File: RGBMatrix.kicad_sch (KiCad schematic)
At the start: 208 parts

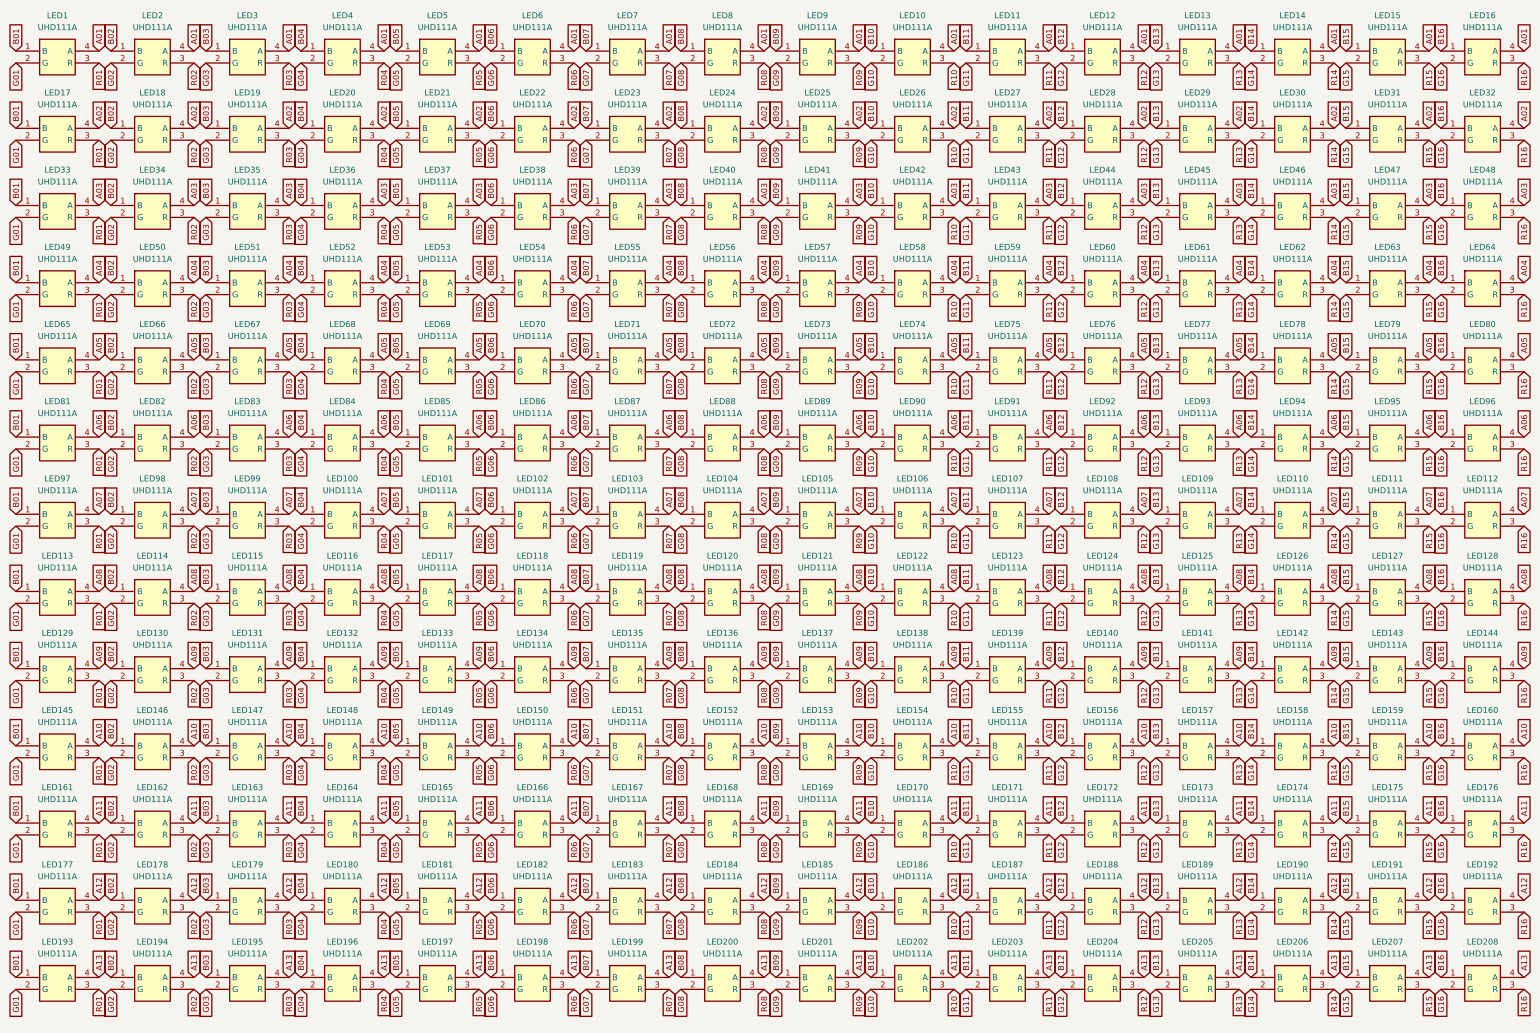
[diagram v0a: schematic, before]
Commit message: anodColumn, colorRow
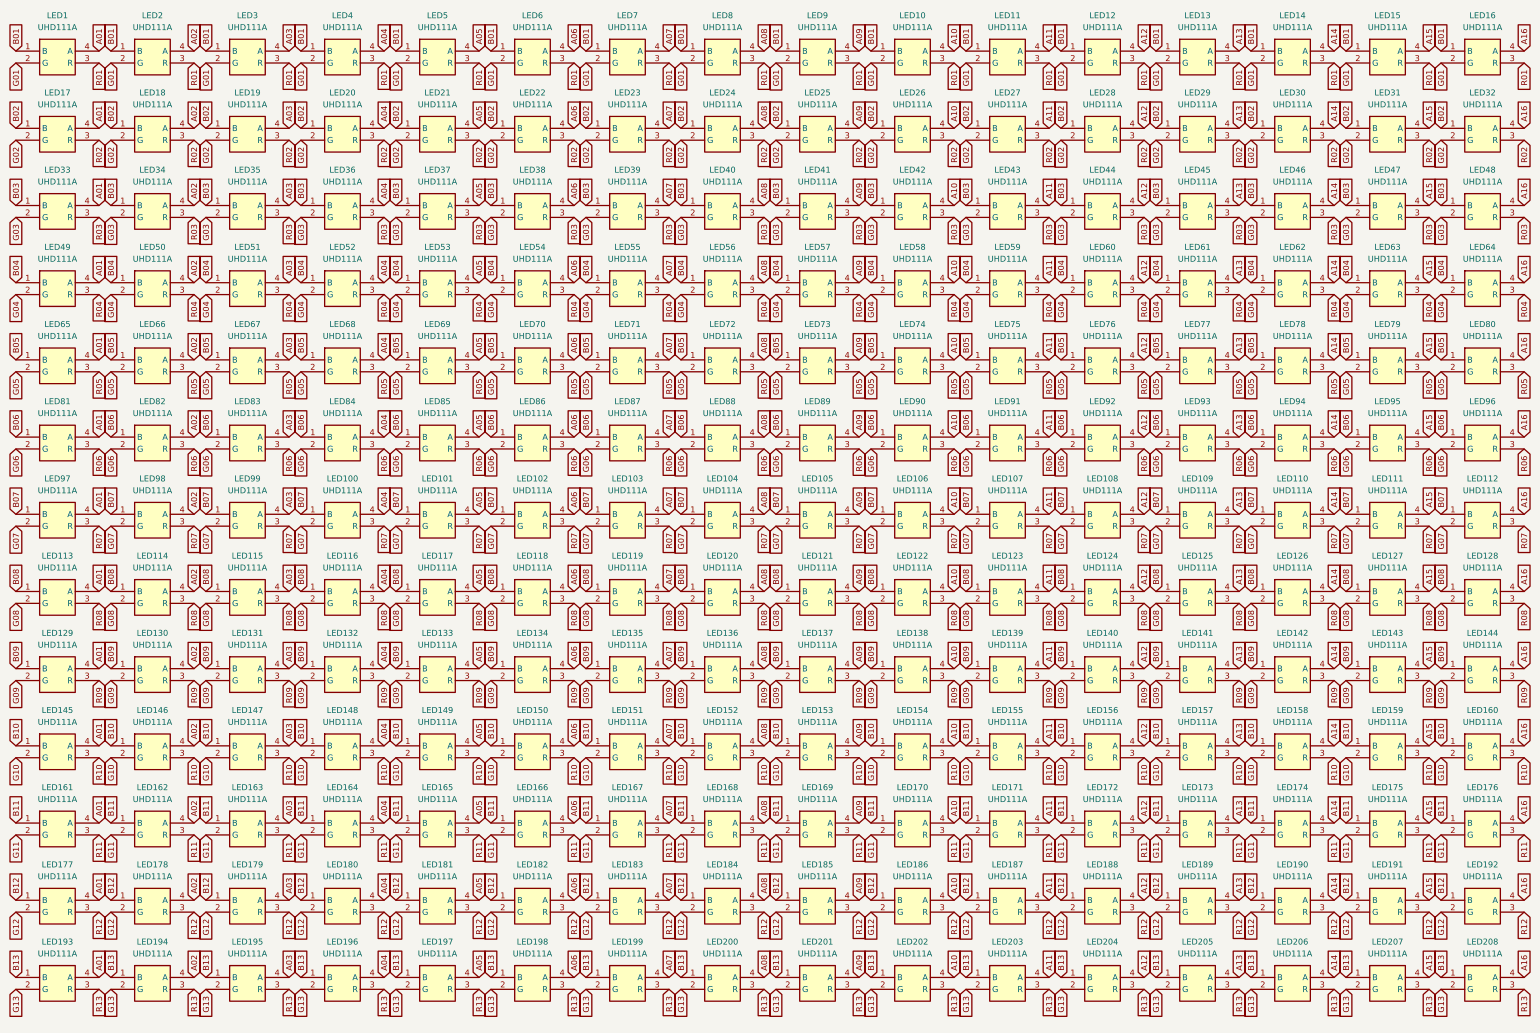
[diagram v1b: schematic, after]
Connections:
- net A01: now also LED113.4 (A), LED129.4 (A), LED145.4 (A), LED161.4 (A), LED17.4 (A), LED177.4 (A), LED193.4 (A), LED33.4 (A), LED49.4 (A), LED65.4 (A), LED81.4 (A), LED97.4 (A); no longer LED10.4 (A), LED11.4 (A), LED12.4 (A), LED13.4 (A), LED14.4 (A), LED15.4 (A), LED16.4 (A), LED2.4 (A), LED3.4 (A), LED4.4 (A), LED5.4 (A), LED6.4 (A), LED7.4 (A), LED8.4 (A), LED9.4 (A)
- net A02: now also LED114.4 (A), LED130.4 (A), LED146.4 (A), LED162.4 (A), LED178.4 (A), LED194.4 (A), LED2.4 (A), LED34.4 (A), LED50.4 (A), LED66.4 (A), LED82.4 (A), LED98.4 (A); no longer LED17.4 (A), LED19.4 (A), LED20.4 (A), LED21.4 (A), LED22.4 (A), LED23.4 (A), LED24.4 (A), LED25.4 (A), LED26.4 (A), LED27.4 (A), LED28.4 (A), LED29.4 (A), LED30.4 (A), LED31.4 (A), LED32.4 (A)
- net A03: now also LED115.4 (A), LED131.4 (A), LED147.4 (A), LED163.4 (A), LED179.4 (A), LED19.4 (A), LED195.4 (A), LED3.4 (A), LED51.4 (A), LED67.4 (A), LED83.4 (A), LED99.4 (A); no longer LED33.4 (A), LED34.4 (A), LED36.4 (A), LED37.4 (A), LED38.4 (A), LED39.4 (A), LED40.4 (A), LED41.4 (A), LED42.4 (A), LED43.4 (A), LED44.4 (A), LED45.4 (A), LED46.4 (A), LED47.4 (A), LED48.4 (A)
- net A04: now also LED100.4 (A), LED116.4 (A), LED132.4 (A), LED148.4 (A), LED164.4 (A), LED180.4 (A), LED196.4 (A), LED20.4 (A), LED36.4 (A), LED4.4 (A), LED68.4 (A), LED84.4 (A); no longer LED49.4 (A), LED50.4 (A), LED51.4 (A), LED53.4 (A), LED54.4 (A), LED55.4 (A), LED56.4 (A), LED57.4 (A), LED58.4 (A), LED59.4 (A), LED60.4 (A), LED61.4 (A), LED62.4 (A), LED63.4 (A), LED64.4 (A)
- net A05: now also LED101.4 (A), LED117.4 (A), LED133.4 (A), LED149.4 (A), LED165.4 (A), LED181.4 (A), LED197.4 (A), LED21.4 (A), LED37.4 (A), LED5.4 (A), LED53.4 (A), LED85.4 (A); no longer LED65.4 (A), LED66.4 (A), LED67.4 (A), LED68.4 (A), LED70.4 (A), LED71.4 (A), LED72.4 (A), LED73.4 (A), LED74.4 (A), LED75.4 (A), LED76.4 (A), LED77.4 (A), LED78.4 (A), LED79.4 (A), LED80.4 (A)
- net A06: now also LED102.4 (A), LED118.4 (A), LED134.4 (A), LED150.4 (A), LED166.4 (A), LED182.4 (A), LED198.4 (A), LED22.4 (A), LED38.4 (A), LED54.4 (A), LED6.4 (A), LED70.4 (A); no longer LED81.4 (A), LED82.4 (A), LED83.4 (A), LED84.4 (A), LED85.4 (A), LED87.4 (A), LED88.4 (A), LED89.4 (A), LED90.4 (A), LED91.4 (A), LED92.4 (A), LED93.4 (A), LED94.4 (A), LED95.4 (A), LED96.4 (A)
- net A07: now also LED119.4 (A), LED135.4 (A), LED151.4 (A), LED167.4 (A), LED183.4 (A), LED199.4 (A), LED23.4 (A), LED39.4 (A), LED55.4 (A), LED7.4 (A), LED71.4 (A), LED87.4 (A); no longer LED100.4 (A), LED101.4 (A), LED102.4 (A), LED104.4 (A), LED105.4 (A), LED106.4 (A), LED107.4 (A), LED108.4 (A), LED109.4 (A), LED110.4 (A), LED111.4 (A), LED112.4 (A), LED97.4 (A), LED98.4 (A), LED99.4 (A)
- net A08: now also LED104.4 (A), LED136.4 (A), LED152.4 (A), LED168.4 (A), LED184.4 (A), LED200.4 (A), LED24.4 (A), LED40.4 (A), LED56.4 (A), LED72.4 (A), LED8.4 (A), LED88.4 (A); no longer LED113.4 (A), LED114.4 (A), LED115.4 (A), LED116.4 (A), LED117.4 (A), LED118.4 (A), LED119.4 (A), LED121.4 (A), LED122.4 (A), LED123.4 (A), LED124.4 (A), LED125.4 (A), LED126.4 (A), LED127.4 (A), LED128.4 (A)
- net A09: now also LED105.4 (A), LED121.4 (A), LED153.4 (A), LED169.4 (A), LED185.4 (A), LED201.4 (A), LED25.4 (A), LED41.4 (A), LED57.4 (A), LED73.4 (A), LED89.4 (A), LED9.4 (A); no longer LED129.4 (A), LED130.4 (A), LED131.4 (A), LED132.4 (A), LED133.4 (A), LED134.4 (A), LED135.4 (A), LED136.4 (A), LED138.4 (A), LED139.4 (A), LED140.4 (A), LED141.4 (A), LED142.4 (A), LED143.4 (A), LED144.4 (A)
- net A10: now also LED10.4 (A), LED106.4 (A), LED122.4 (A), LED138.4 (A), LED170.4 (A), LED186.4 (A), LED202.4 (A), LED26.4 (A), LED42.4 (A), LED58.4 (A), LED74.4 (A), LED90.4 (A); no longer LED145.4 (A), LED146.4 (A), LED147.4 (A), LED148.4 (A), LED149.4 (A), LED150.4 (A), LED151.4 (A), LED152.4 (A), LED153.4 (A), LED155.4 (A), LED156.4 (A), LED157.4 (A), LED158.4 (A), LED159.4 (A), LED160.4 (A)
- net A11: now also LED107.4 (A), LED11.4 (A), LED123.4 (A), LED139.4 (A), LED155.4 (A), LED187.4 (A), LED203.4 (A), LED27.4 (A), LED43.4 (A), LED59.4 (A), LED75.4 (A), LED91.4 (A); no longer LED161.4 (A), LED162.4 (A), LED163.4 (A), LED164.4 (A), LED165.4 (A), LED166.4 (A), LED167.4 (A), LED168.4 (A), LED169.4 (A), LED170.4 (A), LED172.4 (A), LED173.4 (A), LED174.4 (A), LED175.4 (A), LED176.4 (A)
- net A12: now also LED108.4 (A), LED12.4 (A), LED124.4 (A), LED140.4 (A), LED156.4 (A), LED172.4 (A), LED204.4 (A), LED28.4 (A), LED44.4 (A), LED60.4 (A), LED76.4 (A), LED92.4 (A); no longer LED177.4 (A), LED178.4 (A), LED179.4 (A), LED180.4 (A), LED181.4 (A), LED182.4 (A), LED183.4 (A), LED184.4 (A), LED185.4 (A), LED186.4 (A), LED187.4 (A), LED189.4 (A), LED190.4 (A), LED191.4 (A), LED192.4 (A)
- net A13: now also LED109.4 (A), LED125.4 (A), LED13.4 (A), LED141.4 (A), LED157.4 (A), LED173.4 (A), LED189.4 (A), LED29.4 (A), LED45.4 (A), LED61.4 (A), LED77.4 (A), LED93.4 (A); no longer LED193.4 (A), LED194.4 (A), LED195.4 (A), LED196.4 (A), LED197.4 (A), LED198.4 (A), LED199.4 (A), LED200.4 (A), LED201.4 (A), LED202.4 (A), LED203.4 (A), LED204.4 (A), LED206.4 (A), LED207.4 (A), LED208.4 (A)
- net B01: now also LED10.1 (B), LED11.1 (B), LED12.1 (B), LED13.1 (B), LED14.1 (B), LED15.1 (B), LED16.1 (B), LED2.1 (B), LED3.1 (B), LED4.1 (B), LED5.1 (B), LED6.1 (B), LED7.1 (B), LED8.1 (B), LED9.1 (B); no longer LED113.1 (B), LED129.1 (B), LED145.1 (B), LED161.1 (B), LED17.1 (B), LED177.1 (B), LED193.1 (B), LED33.1 (B), LED49.1 (B), LED65.1 (B), LED81.1 (B), LED97.1 (B)
- net B02: now also LED17.1 (B), LED19.1 (B), LED20.1 (B), LED21.1 (B), LED22.1 (B), LED23.1 (B), LED24.1 (B), LED25.1 (B), LED26.1 (B), LED27.1 (B), LED28.1 (B), LED29.1 (B), LED30.1 (B), LED31.1 (B), LED32.1 (B); no longer LED114.1 (B), LED130.1 (B), LED146.1 (B), LED162.1 (B), LED178.1 (B), LED194.1 (B), LED2.1 (B), LED34.1 (B), LED50.1 (B), LED66.1 (B), LED82.1 (B), LED98.1 (B)
- net B03: now also LED33.1 (B), LED34.1 (B), LED36.1 (B), LED37.1 (B), LED38.1 (B), LED39.1 (B), LED40.1 (B), LED41.1 (B), LED42.1 (B), LED43.1 (B), LED44.1 (B), LED45.1 (B), LED46.1 (B), LED47.1 (B), LED48.1 (B); no longer LED115.1 (B), LED131.1 (B), LED147.1 (B), LED163.1 (B), LED179.1 (B), LED19.1 (B), LED195.1 (B), LED3.1 (B), LED51.1 (B), LED67.1 (B), LED83.1 (B), LED99.1 (B)
- net B04: now also LED49.1 (B), LED50.1 (B), LED51.1 (B), LED53.1 (B), LED54.1 (B), LED55.1 (B), LED56.1 (B), LED57.1 (B), LED58.1 (B), LED59.1 (B), LED60.1 (B), LED61.1 (B), LED62.1 (B), LED63.1 (B), LED64.1 (B); no longer LED100.1 (B), LED116.1 (B), LED132.1 (B), LED148.1 (B), LED164.1 (B), LED180.1 (B), LED196.1 (B), LED20.1 (B), LED36.1 (B), LED4.1 (B), LED68.1 (B), LED84.1 (B)
- net B05: now also LED65.1 (B), LED66.1 (B), LED67.1 (B), LED68.1 (B), LED70.1 (B), LED71.1 (B), LED72.1 (B), LED73.1 (B), LED74.1 (B), LED75.1 (B), LED76.1 (B), LED77.1 (B), LED78.1 (B), LED79.1 (B), LED80.1 (B); no longer LED101.1 (B), LED117.1 (B), LED133.1 (B), LED149.1 (B), LED165.1 (B), LED181.1 (B), LED197.1 (B), LED21.1 (B), LED37.1 (B), LED5.1 (B), LED53.1 (B), LED85.1 (B)
- net B06: now also LED81.1 (B), LED82.1 (B), LED83.1 (B), LED84.1 (B), LED85.1 (B), LED87.1 (B), LED88.1 (B), LED89.1 (B), LED90.1 (B), LED91.1 (B), LED92.1 (B), LED93.1 (B), LED94.1 (B), LED95.1 (B), LED96.1 (B); no longer LED102.1 (B), LED118.1 (B), LED134.1 (B), LED150.1 (B), LED166.1 (B), LED182.1 (B), LED198.1 (B), LED22.1 (B), LED38.1 (B), LED54.1 (B), LED6.1 (B), LED70.1 (B)
- net B07: now also LED100.1 (B), LED101.1 (B), LED102.1 (B), LED104.1 (B), LED105.1 (B), LED106.1 (B), LED107.1 (B), LED108.1 (B), LED109.1 (B), LED110.1 (B), LED111.1 (B), LED112.1 (B), LED97.1 (B), LED98.1 (B), LED99.1 (B); no longer LED119.1 (B), LED135.1 (B), LED151.1 (B), LED167.1 (B), LED183.1 (B), LED199.1 (B), LED23.1 (B), LED39.1 (B), LED55.1 (B), LED7.1 (B), LED71.1 (B), LED87.1 (B)
- net B08: now also LED113.1 (B), LED114.1 (B), LED115.1 (B), LED116.1 (B), LED117.1 (B), LED118.1 (B), LED119.1 (B), LED121.1 (B), LED122.1 (B), LED123.1 (B), LED124.1 (B), LED125.1 (B), LED126.1 (B), LED127.1 (B), LED128.1 (B); no longer LED104.1 (B), LED136.1 (B), LED152.1 (B), LED168.1 (B), LED184.1 (B), LED200.1 (B), LED24.1 (B), LED40.1 (B), LED56.1 (B), LED72.1 (B), LED8.1 (B), LED88.1 (B)
- net B09: now also LED129.1 (B), LED130.1 (B), LED131.1 (B), LED132.1 (B), LED133.1 (B), LED134.1 (B), LED135.1 (B), LED136.1 (B), LED138.1 (B), LED139.1 (B), LED140.1 (B), LED141.1 (B), LED142.1 (B), LED143.1 (B), LED144.1 (B); no longer LED105.1 (B), LED121.1 (B), LED153.1 (B), LED169.1 (B), LED185.1 (B), LED201.1 (B), LED25.1 (B), LED41.1 (B), LED57.1 (B), LED73.1 (B), LED89.1 (B), LED9.1 (B)
- net B10: now also LED145.1 (B), LED146.1 (B), LED147.1 (B), LED148.1 (B), LED149.1 (B), LED150.1 (B), LED151.1 (B), LED152.1 (B), LED153.1 (B), LED155.1 (B), LED156.1 (B), LED157.1 (B), LED158.1 (B), LED159.1 (B), LED160.1 (B); no longer LED10.1 (B), LED106.1 (B), LED122.1 (B), LED138.1 (B), LED170.1 (B), LED186.1 (B), LED202.1 (B), LED26.1 (B), LED42.1 (B), LED58.1 (B), LED74.1 (B), LED90.1 (B)
- net B11: now also LED161.1 (B), LED162.1 (B), LED163.1 (B), LED164.1 (B), LED165.1 (B), LED166.1 (B), LED167.1 (B), LED168.1 (B), LED169.1 (B), LED170.1 (B), LED172.1 (B), LED173.1 (B), LED174.1 (B), LED175.1 (B), LED176.1 (B); no longer LED107.1 (B), LED11.1 (B), LED123.1 (B), LED139.1 (B), LED155.1 (B), LED187.1 (B), LED203.1 (B), LED27.1 (B), LED43.1 (B), LED59.1 (B), LED75.1 (B), LED91.1 (B)
- net B12: now also LED177.1 (B), LED178.1 (B), LED179.1 (B), LED180.1 (B), LED181.1 (B), LED182.1 (B), LED183.1 (B), LED184.1 (B), LED185.1 (B), LED186.1 (B), LED187.1 (B), LED189.1 (B), LED190.1 (B), LED191.1 (B), LED192.1 (B); no longer LED108.1 (B), LED12.1 (B), LED124.1 (B), LED140.1 (B), LED156.1 (B), LED172.1 (B), LED204.1 (B), LED28.1 (B), LED44.1 (B), LED60.1 (B), LED76.1 (B), LED92.1 (B)
- net B13: now also LED193.1 (B), LED194.1 (B), LED195.1 (B), LED196.1 (B), LED197.1 (B), LED198.1 (B), LED199.1 (B), LED200.1 (B), LED201.1 (B), LED202.1 (B), LED203.1 (B), LED204.1 (B), LED206.1 (B), LED207.1 (B), LED208.1 (B); no longer LED109.1 (B), LED125.1 (B), LED13.1 (B), LED141.1 (B), LED157.1 (B), LED173.1 (B), LED189.1 (B), LED29.1 (B), LED45.1 (B), LED61.1 (B), LED77.1 (B), LED93.1 (B)
- net G01: now also LED10.2 (G), LED11.2 (G), LED12.2 (G), LED13.2 (G), LED14.2 (G), LED15.2 (G), LED16.2 (G), LED2.2 (G), LED3.2 (G), LED4.2 (G), LED5.2 (G), LED6.2 (G), LED7.2 (G), LED8.2 (G), LED9.2 (G); no longer LED113.2 (G), LED129.2 (G), LED145.2 (G), LED161.2 (G), LED17.2 (G), LED177.2 (G), LED193.2 (G), LED33.2 (G), LED49.2 (G), LED65.2 (G), LED81.2 (G), LED97.2 (G)
- net G02: now also LED17.2 (G), LED19.2 (G), LED20.2 (G), LED21.2 (G), LED22.2 (G), LED23.2 (G), LED24.2 (G), LED25.2 (G), LED26.2 (G), LED27.2 (G), LED28.2 (G), LED29.2 (G), LED30.2 (G), LED31.2 (G), LED32.2 (G); no longer LED114.2 (G), LED130.2 (G), LED146.2 (G), LED162.2 (G), LED178.2 (G), LED194.2 (G), LED2.2 (G), LED34.2 (G), LED50.2 (G), LED66.2 (G), LED82.2 (G), LED98.2 (G)
- net G03: now also LED33.2 (G), LED34.2 (G), LED36.2 (G), LED37.2 (G), LED38.2 (G), LED39.2 (G), LED40.2 (G), LED41.2 (G), LED42.2 (G), LED43.2 (G), LED44.2 (G), LED45.2 (G), LED46.2 (G), LED47.2 (G), LED48.2 (G); no longer LED115.2 (G), LED131.2 (G), LED147.2 (G), LED163.2 (G), LED179.2 (G), LED19.2 (G), LED195.2 (G), LED3.2 (G), LED51.2 (G), LED67.2 (G), LED83.2 (G), LED99.2 (G)
- net G04: now also LED49.2 (G), LED50.2 (G), LED51.2 (G), LED53.2 (G), LED54.2 (G), LED55.2 (G), LED56.2 (G), LED57.2 (G), LED58.2 (G), LED59.2 (G), LED60.2 (G), LED61.2 (G), LED62.2 (G), LED63.2 (G), LED64.2 (G); no longer LED100.2 (G), LED116.2 (G), LED132.2 (G), LED148.2 (G), LED164.2 (G), LED180.2 (G), LED196.2 (G), LED20.2 (G), LED36.2 (G), LED4.2 (G), LED68.2 (G), LED84.2 (G)
- net G05: now also LED65.2 (G), LED66.2 (G), LED67.2 (G), LED68.2 (G), LED70.2 (G), LED71.2 (G), LED72.2 (G), LED73.2 (G), LED74.2 (G), LED75.2 (G), LED76.2 (G), LED77.2 (G), LED78.2 (G), LED79.2 (G), LED80.2 (G); no longer LED101.2 (G), LED117.2 (G), LED133.2 (G), LED149.2 (G), LED165.2 (G), LED181.2 (G), LED197.2 (G), LED21.2 (G), LED37.2 (G), LED5.2 (G), LED53.2 (G), LED85.2 (G)
- net G06: now also LED81.2 (G), LED82.2 (G), LED83.2 (G), LED84.2 (G), LED85.2 (G), LED87.2 (G), LED88.2 (G), LED89.2 (G), LED90.2 (G), LED91.2 (G), LED92.2 (G), LED93.2 (G), LED94.2 (G), LED95.2 (G), LED96.2 (G); no longer LED102.2 (G), LED118.2 (G), LED134.2 (G), LED150.2 (G), LED166.2 (G), LED182.2 (G), LED198.2 (G), LED22.2 (G), LED38.2 (G), LED54.2 (G), LED6.2 (G), LED70.2 (G)
- net G07: now also LED100.2 (G), LED101.2 (G), LED102.2 (G), LED104.2 (G), LED105.2 (G), LED106.2 (G), LED107.2 (G), LED108.2 (G), LED109.2 (G), LED110.2 (G), LED111.2 (G), LED112.2 (G), LED97.2 (G), LED98.2 (G), LED99.2 (G); no longer LED119.2 (G), LED135.2 (G), LED151.2 (G), LED167.2 (G), LED183.2 (G), LED199.2 (G), LED23.2 (G), LED39.2 (G), LED55.2 (G), LED7.2 (G), LED71.2 (G), LED87.2 (G)
- net G08: now also LED113.2 (G), LED114.2 (G), LED115.2 (G), LED116.2 (G), LED117.2 (G), LED118.2 (G), LED119.2 (G), LED121.2 (G), LED122.2 (G), LED123.2 (G), LED124.2 (G), LED125.2 (G), LED126.2 (G), LED127.2 (G), LED128.2 (G); no longer LED104.2 (G), LED136.2 (G), LED152.2 (G), LED168.2 (G), LED184.2 (G), LED200.2 (G), LED24.2 (G), LED40.2 (G), LED56.2 (G), LED72.2 (G), LED8.2 (G), LED88.2 (G)
- net G09: now also LED129.2 (G), LED130.2 (G), LED131.2 (G), LED132.2 (G), LED133.2 (G), LED134.2 (G), LED135.2 (G), LED136.2 (G), LED138.2 (G), LED139.2 (G), LED140.2 (G), LED141.2 (G), LED142.2 (G), LED143.2 (G), LED144.2 (G); no longer LED105.2 (G), LED121.2 (G), LED153.2 (G), LED169.2 (G), LED185.2 (G), LED201.2 (G), LED25.2 (G), LED41.2 (G), LED57.2 (G), LED73.2 (G), LED89.2 (G), LED9.2 (G)
- net G10: now also LED145.2 (G), LED146.2 (G), LED147.2 (G), LED148.2 (G), LED149.2 (G), LED150.2 (G), LED151.2 (G), LED152.2 (G), LED153.2 (G), LED155.2 (G), LED156.2 (G), LED157.2 (G), LED158.2 (G), LED159.2 (G), LED160.2 (G); no longer LED10.2 (G), LED106.2 (G), LED122.2 (G), LED138.2 (G), LED170.2 (G), LED186.2 (G), LED202.2 (G), LED26.2 (G), LED42.2 (G), LED58.2 (G), LED74.2 (G), LED90.2 (G)
- net G11: now also LED161.2 (G), LED162.2 (G), LED163.2 (G), LED164.2 (G), LED165.2 (G), LED166.2 (G), LED167.2 (G), LED168.2 (G), LED169.2 (G), LED170.2 (G), LED172.2 (G), LED173.2 (G), LED174.2 (G), LED175.2 (G), LED176.2 (G); no longer LED107.2 (G), LED11.2 (G), LED123.2 (G), LED139.2 (G), LED155.2 (G), LED187.2 (G), LED203.2 (G), LED27.2 (G), LED43.2 (G), LED59.2 (G), LED75.2 (G), LED91.2 (G)
- net G12: now also LED177.2 (G), LED178.2 (G), LED179.2 (G), LED180.2 (G), LED181.2 (G), LED182.2 (G), LED183.2 (G), LED184.2 (G), LED185.2 (G), LED186.2 (G), LED187.2 (G), LED189.2 (G), LED190.2 (G), LED191.2 (G), LED192.2 (G); no longer LED108.2 (G), LED12.2 (G), LED124.2 (G), LED140.2 (G), LED156.2 (G), LED172.2 (G), LED204.2 (G), LED28.2 (G), LED44.2 (G), LED60.2 (G), LED76.2 (G), LED92.2 (G)
- net G13: now also LED193.2 (G), LED194.2 (G), LED195.2 (G), LED196.2 (G), LED197.2 (G), LED198.2 (G), LED199.2 (G), LED200.2 (G), LED201.2 (G), LED202.2 (G), LED203.2 (G), LED204.2 (G), LED206.2 (G), LED207.2 (G), LED208.2 (G); no longer LED109.2 (G), LED125.2 (G), LED13.2 (G), LED141.2 (G), LED157.2 (G), LED173.2 (G), LED189.2 (G), LED29.2 (G), LED45.2 (G), LED61.2 (G), LED77.2 (G), LED93.2 (G)
- net R01: now also LED10.3 (R), LED11.3 (R), LED12.3 (R), LED13.3 (R), LED14.3 (R), LED15.3 (R), LED16.3 (R), LED2.3 (R), LED3.3 (R), LED4.3 (R), LED5.3 (R), LED6.3 (R), LED7.3 (R), LED8.3 (R), LED9.3 (R); no longer LED113.3 (R), LED129.3 (R), LED145.3 (R), LED161.3 (R), LED17.3 (R), LED177.3 (R), LED193.3 (R), LED33.3 (R), LED49.3 (R), LED65.3 (R), LED81.3 (R), LED97.3 (R)
- net R02: now also LED17.3 (R), LED19.3 (R), LED20.3 (R), LED21.3 (R), LED22.3 (R), LED23.3 (R), LED24.3 (R), LED25.3 (R), LED26.3 (R), LED27.3 (R), LED28.3 (R), LED29.3 (R), LED30.3 (R), LED31.3 (R), LED32.3 (R); no longer LED114.3 (R), LED130.3 (R), LED146.3 (R), LED162.3 (R), LED178.3 (R), LED194.3 (R), LED2.3 (R), LED34.3 (R), LED50.3 (R), LED66.3 (R), LED82.3 (R), LED98.3 (R)
- net R03: now also LED33.3 (R), LED34.3 (R), LED36.3 (R), LED37.3 (R), LED38.3 (R), LED39.3 (R), LED40.3 (R), LED41.3 (R), LED42.3 (R), LED43.3 (R), LED44.3 (R), LED45.3 (R), LED46.3 (R), LED47.3 (R), LED48.3 (R); no longer LED115.3 (R), LED131.3 (R), LED147.3 (R), LED163.3 (R), LED179.3 (R), LED19.3 (R), LED195.3 (R), LED3.3 (R), LED51.3 (R), LED67.3 (R), LED83.3 (R), LED99.3 (R)
- net R04: now also LED49.3 (R), LED50.3 (R), LED51.3 (R), LED53.3 (R), LED54.3 (R), LED55.3 (R), LED56.3 (R), LED57.3 (R), LED58.3 (R), LED59.3 (R), LED60.3 (R), LED61.3 (R), LED62.3 (R), LED63.3 (R), LED64.3 (R); no longer LED100.3 (R), LED116.3 (R), LED132.3 (R), LED148.3 (R), LED164.3 (R), LED180.3 (R), LED196.3 (R), LED20.3 (R), LED36.3 (R), LED4.3 (R), LED68.3 (R), LED84.3 (R)
- net R05: now also LED65.3 (R), LED66.3 (R), LED67.3 (R), LED68.3 (R), LED70.3 (R), LED71.3 (R), LED72.3 (R), LED73.3 (R), LED74.3 (R), LED75.3 (R), LED76.3 (R), LED77.3 (R), LED78.3 (R), LED79.3 (R), LED80.3 (R); no longer LED101.3 (R), LED117.3 (R), LED133.3 (R), LED149.3 (R), LED165.3 (R), LED181.3 (R), LED197.3 (R), LED21.3 (R), LED37.3 (R), LED5.3 (R), LED53.3 (R), LED85.3 (R)
- net R06: now also LED81.3 (R), LED82.3 (R), LED83.3 (R), LED84.3 (R), LED85.3 (R), LED87.3 (R), LED88.3 (R), LED89.3 (R), LED90.3 (R), LED91.3 (R), LED92.3 (R), LED93.3 (R), LED94.3 (R), LED95.3 (R), LED96.3 (R); no longer LED102.3 (R), LED118.3 (R), LED134.3 (R), LED150.3 (R), LED166.3 (R), LED182.3 (R), LED198.3 (R), LED22.3 (R), LED38.3 (R), LED54.3 (R), LED6.3 (R), LED70.3 (R)
- net R07: now also LED100.3 (R), LED101.3 (R), LED102.3 (R), LED104.3 (R), LED105.3 (R), LED106.3 (R), LED107.3 (R), LED108.3 (R), LED109.3 (R), LED110.3 (R), LED111.3 (R), LED112.3 (R), LED97.3 (R), LED98.3 (R), LED99.3 (R); no longer LED119.3 (R), LED135.3 (R), LED151.3 (R), LED167.3 (R), LED183.3 (R), LED199.3 (R), LED23.3 (R), LED39.3 (R), LED55.3 (R), LED7.3 (R), LED71.3 (R), LED87.3 (R)
- net R08: now also LED113.3 (R), LED114.3 (R), LED115.3 (R), LED116.3 (R), LED117.3 (R), LED118.3 (R), LED119.3 (R), LED121.3 (R), LED122.3 (R), LED123.3 (R), LED124.3 (R), LED125.3 (R), LED126.3 (R), LED127.3 (R), LED128.3 (R); no longer LED104.3 (R), LED136.3 (R), LED152.3 (R), LED168.3 (R), LED184.3 (R), LED200.3 (R), LED24.3 (R), LED40.3 (R), LED56.3 (R), LED72.3 (R), LED8.3 (R), LED88.3 (R)
- net R09: now also LED129.3 (R), LED130.3 (R), LED131.3 (R), LED132.3 (R), LED133.3 (R), LED134.3 (R), LED135.3 (R), LED136.3 (R), LED138.3 (R), LED139.3 (R), LED140.3 (R), LED141.3 (R), LED142.3 (R), LED143.3 (R), LED144.3 (R); no longer LED105.3 (R), LED121.3 (R), LED153.3 (R), LED169.3 (R), LED185.3 (R), LED201.3 (R), LED25.3 (R), LED41.3 (R), LED57.3 (R), LED73.3 (R), LED89.3 (R), LED9.3 (R)
- net R10: now also LED145.3 (R), LED146.3 (R), LED147.3 (R), LED148.3 (R), LED149.3 (R), LED150.3 (R), LED151.3 (R), LED152.3 (R), LED153.3 (R), LED155.3 (R), LED156.3 (R), LED157.3 (R), LED158.3 (R), LED159.3 (R), LED160.3 (R); no longer LED10.3 (R), LED106.3 (R), LED122.3 (R), LED138.3 (R), LED170.3 (R), LED186.3 (R), LED202.3 (R), LED26.3 (R), LED42.3 (R), LED58.3 (R), LED74.3 (R), LED90.3 (R)
- net R11: now also LED161.3 (R), LED162.3 (R), LED163.3 (R), LED164.3 (R), LED165.3 (R), LED166.3 (R), LED167.3 (R), LED168.3 (R), LED169.3 (R), LED170.3 (R), LED172.3 (R), LED173.3 (R), LED174.3 (R), LED175.3 (R), LED176.3 (R); no longer LED107.3 (R), LED11.3 (R), LED123.3 (R), LED139.3 (R), LED155.3 (R), LED187.3 (R), LED203.3 (R), LED27.3 (R), LED43.3 (R), LED59.3 (R), LED75.3 (R), LED91.3 (R)
- net R12: now also LED177.3 (R), LED178.3 (R), LED179.3 (R), LED180.3 (R), LED181.3 (R), LED182.3 (R), LED183.3 (R), LED184.3 (R), LED185.3 (R), LED186.3 (R), LED187.3 (R), LED189.3 (R), LED190.3 (R), LED191.3 (R), LED192.3 (R); no longer LED108.3 (R), LED12.3 (R), LED124.3 (R), LED140.3 (R), LED156.3 (R), LED172.3 (R), LED204.3 (R), LED28.3 (R), LED44.3 (R), LED60.3 (R), LED76.3 (R), LED92.3 (R)
- net R13: now also LED193.3 (R), LED194.3 (R), LED195.3 (R), LED196.3 (R), LED197.3 (R), LED198.3 (R), LED199.3 (R), LED200.3 (R), LED201.3 (R), LED202.3 (R), LED203.3 (R), LED204.3 (R), LED206.3 (R), LED207.3 (R), LED208.3 (R); no longer LED109.3 (R), LED125.3 (R), LED13.3 (R), LED141.3 (R), LED157.3 (R), LED173.3 (R), LED189.3 (R), LED29.3 (R), LED45.3 (R), LED61.3 (R), LED77.3 (R), LED93.3 (R)
- removed net B14: LED110.1 (B), LED126.1 (B), LED14.1 (B), LED142.1 (B), LED158.1 (B), LED174.1 (B), LED190.1 (B), LED206.1 (B), LED30.1 (B), LED46.1 (B), LED62.1 (B), LED78.1 (B), LED94.1 (B)
- removed net B15: LED111.1 (B), LED127.1 (B), LED143.1 (B), LED15.1 (B), LED159.1 (B), LED175.1 (B), LED191.1 (B), LED207.1 (B), LED31.1 (B), LED47.1 (B), LED63.1 (B), LED79.1 (B), LED95.1 (B)
- removed net B16: LED112.1 (B), LED128.1 (B), LED144.1 (B), LED16.1 (B), LED160.1 (B), LED176.1 (B), LED192.1 (B), LED208.1 (B), LED32.1 (B), LED48.1 (B), LED64.1 (B), LED80.1 (B), LED96.1 (B)
- removed net G14: LED110.2 (G), LED126.2 (G), LED14.2 (G), LED142.2 (G), LED158.2 (G), LED174.2 (G), LED190.2 (G), LED206.2 (G), LED30.2 (G), LED46.2 (G), LED62.2 (G), LED78.2 (G), LED94.2 (G)
- removed net G15: LED111.2 (G), LED127.2 (G), LED143.2 (G), LED15.2 (G), LED159.2 (G), LED175.2 (G), LED191.2 (G), LED207.2 (G), LED31.2 (G), LED47.2 (G), LED63.2 (G), LED79.2 (G), LED95.2 (G)
- removed net G16: LED112.2 (G), LED128.2 (G), LED144.2 (G), LED16.2 (G), LED160.2 (G), LED176.2 (G), LED192.2 (G), LED208.2 (G), LED32.2 (G), LED48.2 (G), LED64.2 (G), LED80.2 (G), LED96.2 (G)
- removed net R14: LED110.3 (R), LED126.3 (R), LED14.3 (R), LED142.3 (R), LED158.3 (R), LED174.3 (R), LED190.3 (R), LED206.3 (R), LED30.3 (R), LED46.3 (R), LED62.3 (R), LED78.3 (R), LED94.3 (R)
- removed net R15: LED111.3 (R), LED127.3 (R), LED143.3 (R), LED15.3 (R), LED159.3 (R), LED175.3 (R), LED191.3 (R), LED207.3 (R), LED31.3 (R), LED47.3 (R), LED63.3 (R), LED79.3 (R), LED95.3 (R)
- removed net R16: LED112.3 (R), LED128.3 (R), LED144.3 (R), LED16.3 (R), LED160.3 (R), LED176.3 (R), LED192.3 (R), LED208.3 (R), LED32.3 (R), LED48.3 (R), LED64.3 (R), LED80.3 (R), LED96.3 (R)
- new net A14: LED110.4 (A), LED126.4 (A), LED14.4 (A), LED142.4 (A), LED158.4 (A), LED174.4 (A), LED190.4 (A), LED206.4 (A), LED30.4 (A), LED46.4 (A), LED62.4 (A), LED78.4 (A), LED94.4 (A)
- new net A15: LED111.4 (A), LED127.4 (A), LED143.4 (A), LED15.4 (A), LED159.4 (A), LED175.4 (A), LED191.4 (A), LED207.4 (A), LED31.4 (A), LED47.4 (A), LED63.4 (A), LED79.4 (A), LED95.4 (A)
- new net A16: LED112.4 (A), LED128.4 (A), LED144.4 (A), LED16.4 (A), LED160.4 (A), LED176.4 (A), LED192.4 (A), LED208.4 (A), LED32.4 (A), LED48.4 (A), LED64.4 (A), LED80.4 (A), LED96.4 (A)
